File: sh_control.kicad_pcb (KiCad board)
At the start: 4 copper layers, 86.4 x 94.7 mm, 90 parts, among them IC1 SN75240PW, IC2 LM317MDCY, IC3 TPS73533DRBT, IC4 TLV76733DGNR, IC5 TUSB2046IBVF, IC6 TPS2044BDR, IC7 SN75240PW, J1 USB_B_Micro, J2 10129381-906001BLF, J3 10129381-906001BLF, SW1 Reset, Y1 6MHz

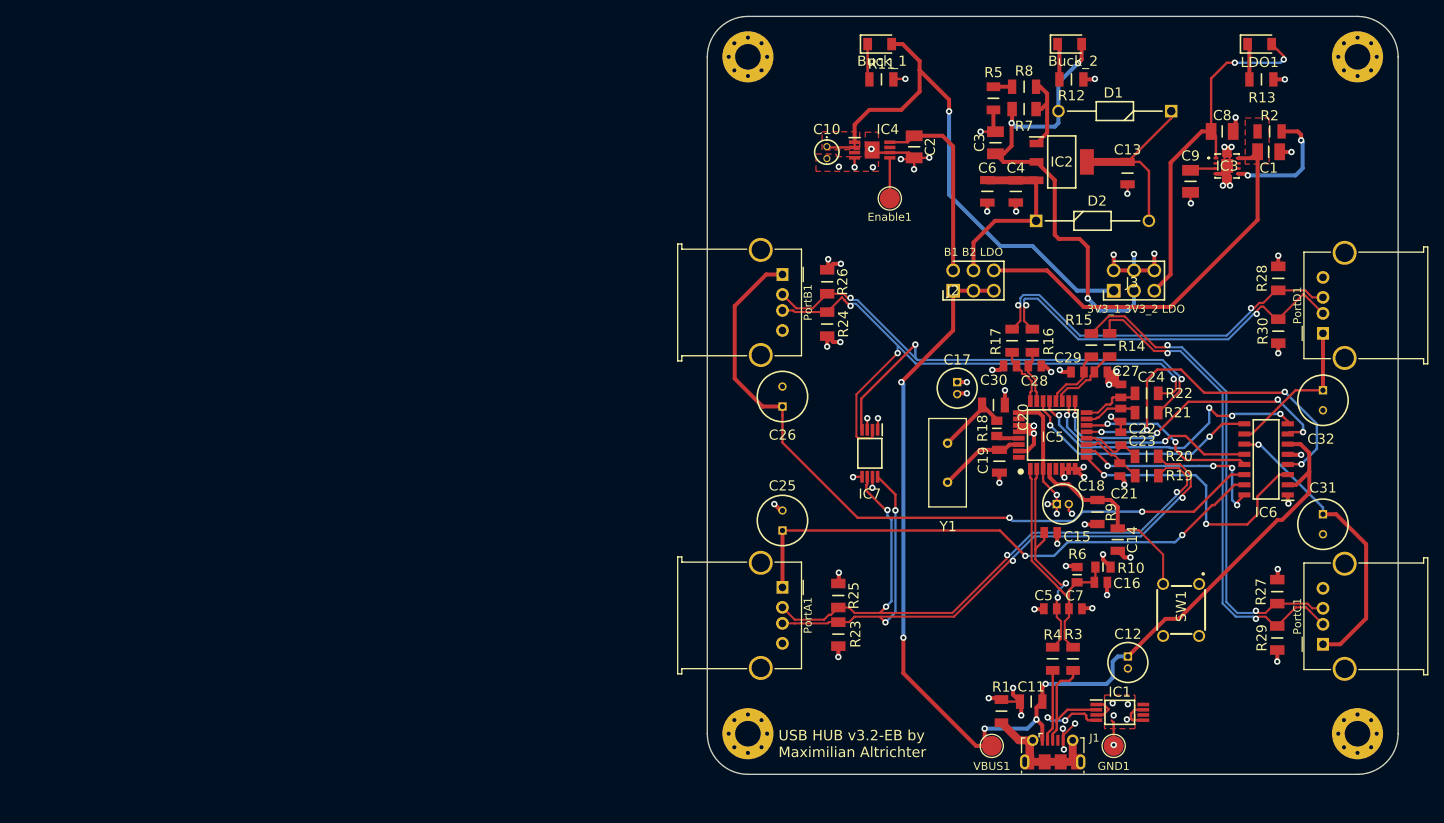
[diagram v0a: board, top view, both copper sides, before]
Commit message: start V3.3
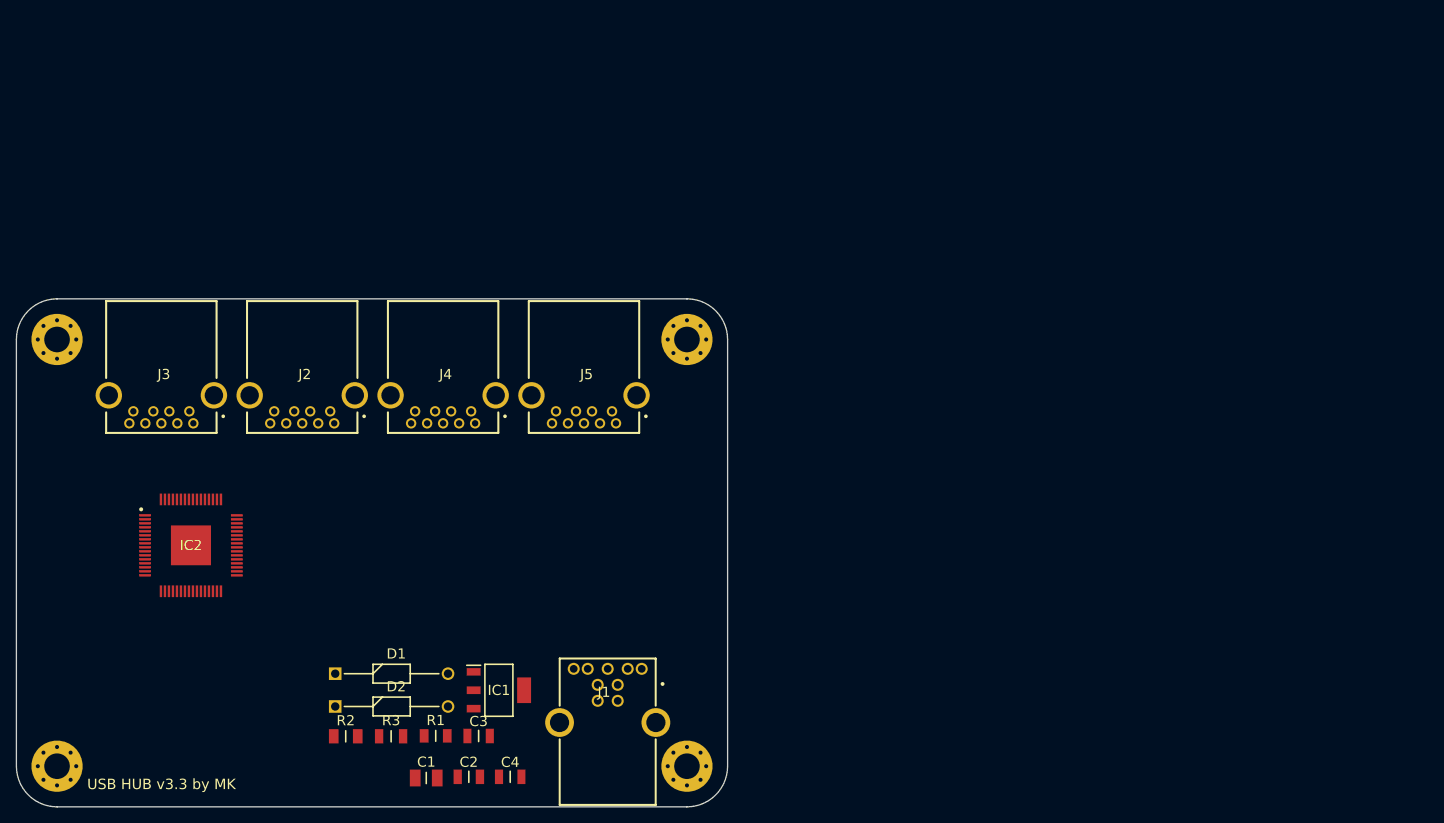
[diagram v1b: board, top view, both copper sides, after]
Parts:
- removed Buck_1: Buck_1, SamacSys_Parts:LEDC3214X78N
- removed Buck_2: Buck_2, SamacSys_Parts:LEDC3214X78N
- removed C10: 2.2uF, storage:C_2.2F
- removed C11, C13, C14, C6: 0.1uF, storage:C_0.1uF
- removed C12, C17, C18: 4.7uF, storage:C_4.7uF
- removed C15, C16, C21, C22, C23, C24, C27, C28, C29, C30, C5, C7: 22pF, storage:C_22pF
- removed C19, C20: 27uF, storage:C_27pF
- removed C25, C26, C31, C32: 100uF, storage:C_100uF
- removed C8, C9: 1uF, storage:C_1uF
- removed Enable1: TestPoint, TestPoint:TestPoint_Pad_D2.5mm
- removed GND1: GND, TestPoint:TestPoint_Pad_D2.5mm
- removed IC3: TPS73533DRBT, SamacSys_Parts:TPS73533DRBT
- removed IC4: TLV76733DGNR, SamacSys_Parts:SOP65P490X110-9N
- removed IC5: TUSB2046IBVF, SamacSys_Parts:QFP80P900X900X160-32N
- removed IC6: TPS2044BDR, SamacSys_Parts:SOIC127P600X175-16N
- removed IC7: SN75240PW, SamacSys_Parts:SOP65P640X120-8N
- removed LDO1: LDO, SamacSys_Parts:LEDC3214X78N
- removed PortA1, PortB1, PortC1, PortD1: USB_A, Connector_USB:USB_A_Molex_67643_Horizontal
- removed R10, R18, R6: 1.5k, storage:R_1K5
- removed R11, R12, R13: 1k, storage:R_1K
- removed R14, R15, R16, R17, R19, R20, R21, R22, R4, R5: 22, storage:R_22
- removed R23, R24, R25, R26, R27, R28, R29, R30: 15k, storage:R_15K
- removed R7: 240, storage:R_240
- removed R8: 390, storage:R_390
- removed R9: 10k, storage:R_10K
- removed SW1: Reset, SamacSys_Parts:FSM4JH
- removed VBUS1: VBUS, TestPoint:TestPoint_Pad_D2.5mm
- removed Y1: 6MHz, SamacSys_Parts:LFXTAL036567BULK
- added J4: 692121030100, SamacSys_Parts:692121030100, F.Cu at (85.6, 68.9)
- added J5: 692121030100, SamacSys_Parts:692121030100, F.Cu at (103.3, 68.9)
- C2: value 1uF -> 10uF; footprint storage:C_1uF -> storage:C_10uF
- C3: value 1uF -> 0.1uF; footprint storage:C_1uF -> storage:C_0.1uF
- C4: value 10uF -> 0.1uF; footprint storage:C_10uF -> storage:C_0.1uF
- IC1: value SN75240PW -> LM317MDCY; footprint SamacSys_Parts:SOP65P640X120-8N -> SamacSys_Parts:SOT230P700X180-4N
- IC2: value LM317MDCY -> TUSB8041IPAPRQ1; footprint SamacSys_Parts:SOT230P700X180-4N -> SamacSys_Parts:QFP50P1200X1200X120-65N
- J1: value USB_B_Micro -> 692221030100; footprint Connector_USB:USB_Micro-B_Molex-105017-0001 -> SamacSys_Parts:WR-COM_USB_TYPE_B
- J2, J3: value 10129381-906001BLF -> 692121030100; footprint SamacSys_Parts:HDRV6W67P254_2X3_762X483X858P -> SamacSys_Parts:692121030100
- R2: value 390 -> 240; footprint storage:R_390 -> storage:R_240
- R3: value 22 -> 390; footprint storage:R_22 -> storage:R_390
- moved R2 138.0 mm to (66.6, 123.3)
- moved C1 131.2 mm to (76.6, 128.5)
- moved D1 126.0 mm to (65.3, 115.4), turned to 0 degrees
- moved H2 123.8 mm to (30.5, 127.0)
- moved IC2 118.9 mm to (47.2, 99.4)
- moved J3 112.1 mm to (50.4, 68.9), turned to 180 degrees
- moved D2 106.6 mm to (65.3, 119.5)
- moved H4 99.4 mm to (30.5, 73.7)
- moved C3 98.4 mm to (83.2, 123.2), turned to 0 degrees
- moved C4 96.7 mm to (87.1, 128.3), turned to 0 degrees
- moved C2 96.4 mm to (82.0, 128.3), turned to 0 degrees
- moved H3 91.0 mm to (109.2, 73.7)
- moved R3 85.8 mm to (72.2, 123.3), turned to 0 degrees
- moved H1 83.9 mm to (109.2, 127.0)
- moved IC1 77.7 mm to (85.7, 117.5)
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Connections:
- C1 pad 1: LDO -> Net-(C1-Pad1)
- C2 pad 1: Buck_1 -> Net-(C2-Pad1)
- C3 pad 1: 3V3_Buck_2 -> Net-(C2-Pad1)
- C4 pad 1: Buck_2 -> Net-(C4-Pad1)
- D1 pad 1: Net-(C13-Pad1) -> Net-(C4-Pad1)
- D1 pad 2: 3V3_Buck_2 -> Net-(C1-Pad1)
- D2 pad 1: Buck_2 -> Net-(C2-Pad1)
- D2 pad 2: Net-(C13-Pad1) -> Net-(C4-Pad1)
- IC1 pad 1: GND -> Net-(IC1-Pad1)
- IC1 pad 2: Net-(IC1-Pad2) -> Net-(C1-Pad1)
- IC1 pad 3: GND -> Net-(C2-Pad1)
- IC1 pad 4: Net-(IC1-Pad4) -> Net-(C4-Pad1)
- IC2 pad 1: Net-(IC2-Pad1) -> (no net)
- IC2 pad 2: 3V3_Buck_2 -> (no net)
- IC2 pad 3: Buck_2 -> (no net)
- IC2 pad 4: Net-(C13-Pad1) -> (no net)
- J1 pad 1: VBUS -> (no net)
- J1 pad 2: Net-(IC1-Pad4) -> (no net)
- J1 pad 3: Net-(IC1-Pad2) -> (no net)
- J1 pad 5: GND -> (no net)
- J1 pad 6: Net-(J1-Pad6) -> (no net)
- J2 pad 1: VBUS -> (no net)
- J2 pad 2: Buck_1 -> (no net)
- J2 pad 3: VBUS -> (no net)
- J2 pad 4: Buck_2 -> (no net)
- J2 pad 5: VBUS -> (no net)
- J2 pad 6: LDO -> (no net)
- J3 pad 1: 3V3_Buck_1 -> (no net)
- J3 pad 2: VCC -> (no net)
- J3 pad 3: 3V3_Buck_2 -> (no net)
- J3 pad 4: VCC -> (no net)
- J3 pad 5: 3V3_LDO -> (no net)
- J3 pad 6: VCC -> (no net)
- R1 pad 2: Net-(J1-Pad6) -> Net-(R1-Pad2)
- R2 pad 1: LDO -> Net-(C1-Pad1)
- R2 pad 2: Net-(IC3-Pad5) -> Net-(IC1-Pad1)
- R3 pad 1: D0+ -> Net-(R1-Pad2)
- R3 pad 2: Net-(IC1-Pad2) -> Net-(IC1-Pad1)
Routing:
- net GND: track 151.4 -> 0.00 mm, vias 71 -> 0
- net VBUS: track 143.3 -> 0.00 mm, vias 5 -> 0
- net OUT2: track 92.8 -> 0.00 mm, vias 2 -> 0
- net D_DS_1_+: track 85.6 -> 0.00 mm, vias 4 -> 0
- net D_DS_1_-: track 83.8 -> 0.00 mm, vias 4 -> 0
- net D_DS_2_-: track 76.7 -> 0.00 mm, vias 3 -> 0
- net D_DS_2_+: track 74.8 -> 0.00 mm, vias 3 -> 0
- net OUT1: track 69.8 -> 0.00 mm, vias 2 -> 0
- net 3V3_Buck_1: track 67.0 -> 0.00 mm, vias 1 -> 0
- net D_DS_3_-: track 61.8 -> 0.00 mm, vias 2 -> 0
- net D_DS_3_+: track 61.8 -> 0.00 mm, vias 2 -> 0
- net 3V3_Buck_2: track 59.6 -> 0.00 mm, vias 3 -> 0
- net LDO: track 50.6 -> 0.00 mm
- net D_DS_4_-: track 48.7 -> 0.00 mm, vias 2 -> 0
- net D_DS_4_+: track 47.6 -> 0.00 mm, vias 2 -> 0
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- removed copper zone on F.Cu, net 3V3_Buck_1
- removed copper zone on F.Cu, net GND
- removed copper zone on In1.Cu, net GND
- removed copper zone on F.Cu, net LDO
- removed copper zone on In2.Cu, net VCC
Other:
- board size 86.4 x 94.7 mm -> 88.9 x 63.5 mm
- board text added: "USB HUB v3.3 by MK"
- board text removed: "3V3_1 3V3_2 LDO"
- board text removed: "B1 B2 LDO"
- board text removed: "USB HUB v3.2-EB by Maximilian Altrichter"
